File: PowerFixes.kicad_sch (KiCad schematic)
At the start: 4 parts

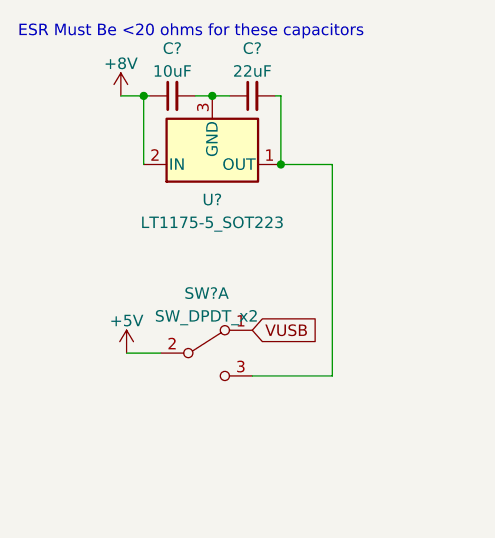
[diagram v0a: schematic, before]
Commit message: Merged in everyone's schematic changes
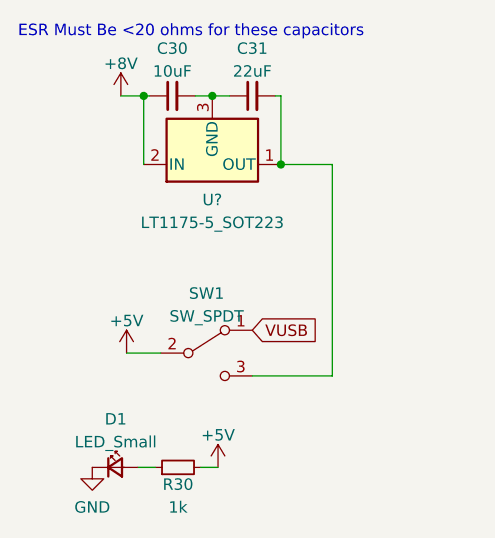
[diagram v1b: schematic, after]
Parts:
- removed SW?: SW_DPDT_x2, symbol Switch:SW_DPDT_x2
- added D1: LED_Small, symbol Device:LED_Small
- added R30: 1k, symbol Device:R_Small
- added SW1: SW_SPDT, symbol Switch:SW_SPDT
- gave numbers to parts that had none: 2
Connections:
- net +5V: now also R30.2, SW1.2 (B)
- net VUSB: now also SW1.1 (A)
- net at C31.2, U?.1 (OUT): now also SW1.3 (C)
- new net: D1.2 (A), R30.1
- new net GND: D1.1 (K)
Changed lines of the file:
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@@
+    (stroke (width 0) (type default) (color 0 0 0 0))
+  )
+  (wire (pts (xy 36.83 66.675) (xy 38.735 66.675))
     (stroke (width 0) (type default) (color 0 0 0 0))
   )
@@
     (stroke (width 0) (type default) (color 0 0 0 0))
   )
+  (wire (pts (xy 29.845 66.675) (xy 31.75 66.675))
+    (stroke (width 0) (type default) (color 0 0 0 0))
+  )
   (text "ESR Must Be <20 ohms for these capacitors" (at 16.51 19.05 0)
     (effects (font (size 1.27 1.27)) (justify left bottom))
@@
     )
   )
-  (symbol (lib_id "Switch:SW_DPDT_x2") (at 37.465 53.975 0) (unit 1)
+  (symbol (lib_id "Device:LED_Small") (at 27.305 66.675 0) (unit 1)
     (in_bom yes) (on_board yes) (fields_autoplaced)
-    (property "Reference" "SW?" (id 0) (at 37.465 47.3542 0))
-    (property "Value" "SW_DPDT_x2" (id 1) (at 37.465 49.8911 0))
-    (property "Footprint" "" (id 2) (at 37.465 53.975 0)
+    (property "Reference" "D1" (id 0) (at 27.3685 61.3242 0))
+    (property "Value" "LED_Small" (id 1) (at 27.3685 63.8611 0))
+    (property "Footprint" "" (id 2) (at 27.305 66.675 90)
       (effects (font (size 1.27 1.27)) hide)
     )
-    (property "Datasheet" "~" (id 3) (at 37.465 53.975 0)
+    (property "Datasheet" "~" (id 3) (at 27.305 66.675 90)
       (effects (font (size 1.27 1.27)) hide)
     )
     (pin "1")
     (pin "2")
-    (pin "3")
-    (pin "4")
-    (pin "5")
-    (pin "6")
   )
   (symbol (lib_id "Device:C_Small") (at 33.655 25.4 90) (unit 1)
     (in_bom yes) (on_board yes)
-    (property "Reference" "C?" (id 0) (at 33.6613 20.1381 90))
+    (property "Reference" "C30" (id 0) (at 33.6613 20.1381 90))
     (property "Value" "10uF" (id 1) (at 33.6613 22.675 90))
     (property "Footprint" "" (id 2) (at 33.655 25.4 0)
@@
   (symbol (lib_id "Device:C_Small") (at 42.545 25.4 90) (unit 1)
     (in_bom yes) (on_board yes) (fields_autoplaced)
-    (property "Reference" "C?" (id 0) (at 42.5513 20.1381 90))
+    (property "Reference" "C31" (id 0) (at 42.5513 20.1381 90))
     (property "Value" "22uF" (id 1) (at 42.5513 22.675 90))
     (property "Footprint" "" (id 2) (at 42.545 25.4 0)
@@
     (pin "1")
   )
+  (symbol (lib_id "power:+5V") (at 38.735 66.675 0) (unit 1)
+    (in_bom yes) (on_board yes) (fields_autoplaced)
+    (property "Reference" "#PWR?" (id 0) (at 38.735 70.485 0)
+      (effects (font (size 1.27 1.27)) hide)
+    )
+    (property "Value" "+5V" (id 1) (at 38.735 63.0992 0))
+    (property "Footprint" "" (id 2) (at 38.735 66.675 0)
+      (effects (font (size 1.27 1.27)) hide)
+    )
+    (property "Datasheet" "" (id 3) (at 38.735 66.675 0)
+      (effects (font (size 1.27 1.27)) hide)
+    )
+    (pin "1")
+  )
+  (symbol (lib_id "Device:R_Small") (at 34.29 66.675 90) (unit 1)
+    (in_bom yes) (on_board yes)
+    (property "Reference" "R30" (id 0) (at 34.29 68.58 90))
+    (property "Value" "1k" (id 1) (at 34.29 71.1169 90))
+    (property "Footprint" "" (id 2) (at 34.29 66.675 0)
+      (effects (font (size 1.27 1.27)) hide)
+    )
+    (property "Datasheet" "~" (id 3) (at 34.29 66.675 0)
+      (effects (font (size 1.27 1.27)) hide)
+    )
+    (pin "1")
+    (pin "2")
+  )
+  (symbol (lib_id "power:GND") (at 24.765 66.675 0) (unit 1)
+    (in_bom yes) (on_board yes) (fields_autoplaced)
+    (property "Reference" "#PWR?" (id 0) (at 24.765 73.025 0)
+      (effects (font (size 1.27 1.27)) hide)
+    )
+    (property "Value" "GND" (id 1) (at 24.765 71.1184 0))
+    (property "Footprint" "" (id 2) (at 24.765 66.675 0)
+      (effects (font (size 1.27 1.27)) hide)
+    )
+    (property "Datasheet" "" (id 3) (at 24.765 66.675 0)
+      (effects (font (size 1.27 1.27)) hide)
+    )
+    (pin "1")
+  )
+  (symbol (lib_id "Switch:SW_SPDT") (at 37.465 53.975 0) (unit 1)
+    (in_bom yes) (on_board yes) (fields_autoplaced)
+    (property "Reference" "SW1" (id 0) (at 37.465 47.3542 0))
+    (property "Value" "SW_SPDT" (id 1) (at 37.465 49.8911 0))
+    (property "Footprint" "" (id 2) (at 37.465 53.975 0)
+      (effects (font (size 1.27 1.27)) hide)
+    )
+    (property "Datasheet" "~" (id 3) (at 37.465 53.975 0)
+      (effects (font (size 1.27 1.27)) hide)
+    )
+    (pin "1")
+    (pin "2")
+    (pin "3")
+  )
   (symbol (lib_id "power:+8V") (at 27.94 25.4 0) (unit 1)
